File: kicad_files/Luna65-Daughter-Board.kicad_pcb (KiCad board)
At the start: 2 copper layers, 25.1 x 25.1 mm, 29 parts, among them J1 TYPE-C-31-M12_13, J2 Molex Power, J3 JSTPH, J4 Conn_01x03, U1 MCP73831, U2 USBLC6-2SC6, U3 AP2112

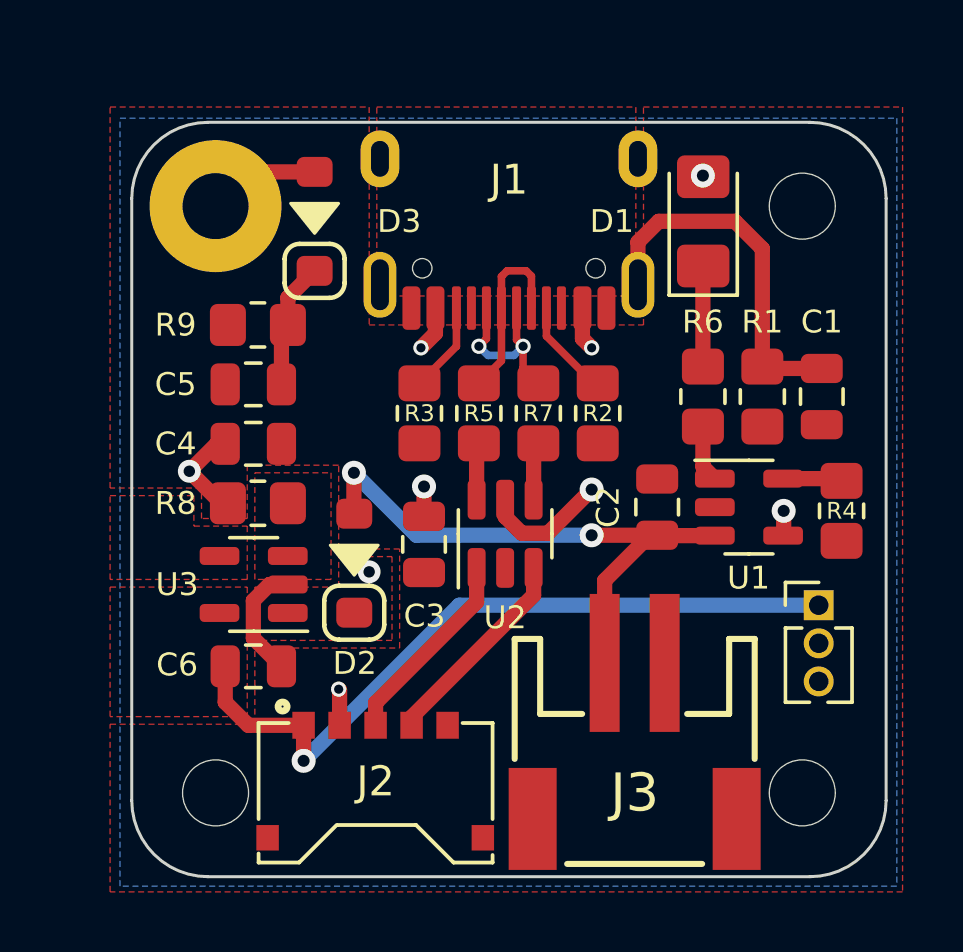
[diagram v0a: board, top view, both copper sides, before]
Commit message: DB Rev B
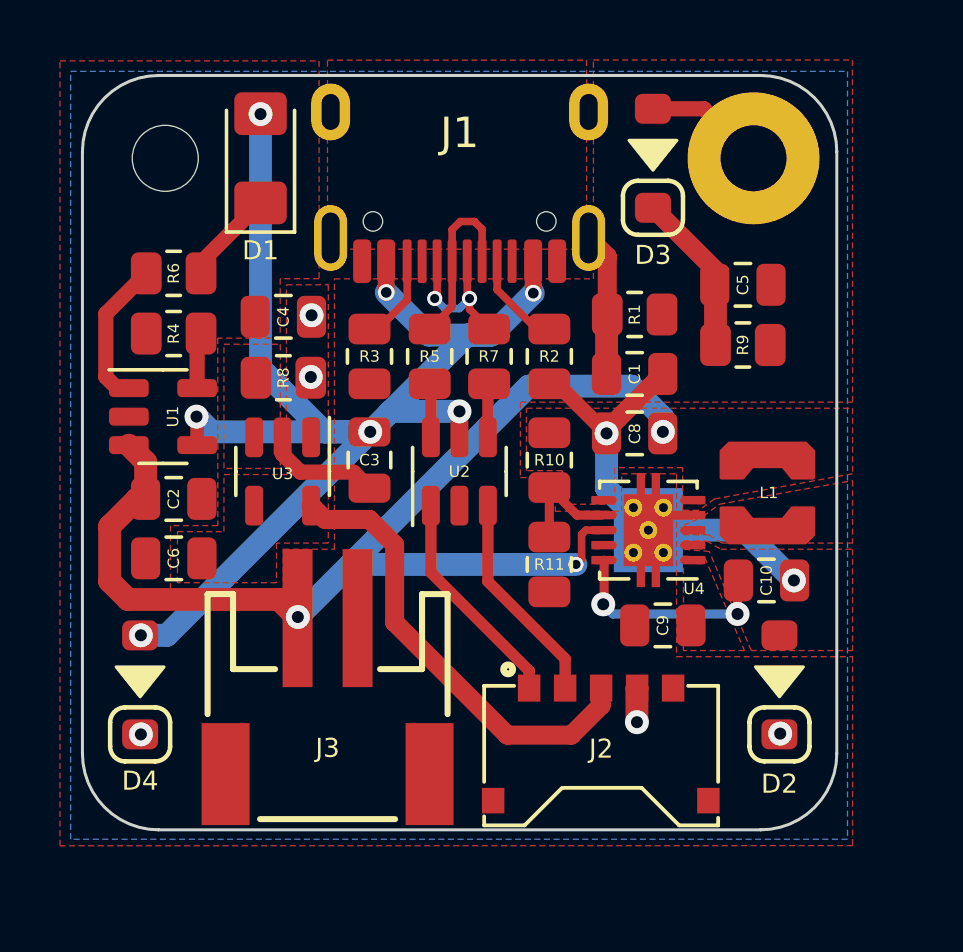
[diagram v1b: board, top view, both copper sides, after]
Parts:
- removed H2, H3: MountingHole, MountingHole:MountingHole_2.2mm_M2
- removed J4: Conn_01x03, Connector_PinHeader_1.27mm:PinHeader_1x03_P1.27mm_Vertical
- added C10: 22uF, acheron_Components:C_0805_2012Metric, F.Cu at (83.5, 37.6)
- added C8: 10uF, acheron_Components:C_0805_2012Metric, F.Cu at (79.1, 32.7)
- added C9: 1uF, acheron_Components:C_0805_2012Metric, F.Cu at (80.0, 39.1)
- added D4: MBR120, acheron_Components:D_SOD-123, F.Cu at (62.6, 41.1)
- added L1: LPS3015-222ML, Luna65:LPS3015, F.Cu at (83.6, 34.7)
- added R10: 3.6M, Resistor_SMD:R_0805_2012Metric, F.Cu at (76.3, 33.6)
- added R11: 261K, Resistor_SMD:R_0805_2012Metric, F.Cu at (76.3, 37.1)
- added U4: TPS61202DRC, Package_SON:Texas_S-PVSON-N10_ThermalVias, F.Cu at (79.6, 36.0)
- R1, R2, R3, R4, R5, R6, R7, R8, R9: footprint Resistor_SMD:R_0805_2012Metric_Pad1.20x1.40mm_HandSolder -> Resistor_SMD:R_0805_2012Metric
- moved R4 23.0 mm to (63.7, 29.4), turned to 180 degrees
- moved H1 21.3 mm to (63.4, 23.6)
- moved U1 19.8 mm to (63.4, 32.2)
- moved R6 18.1 mm to (63.7, 27.4), turned to 0 degrees
- moved H4 18.0 mm to (83.1, 23.6)
- moved C5 16.7 mm to (82.7, 27.8), turned to 0 degrees
- moved R9 16.2 mm to (82.7, 29.8), turned to 180 degrees
- moved C2 16.1 mm to (63.7, 34.9), turned to 180 degrees
- moved D1 14.9 mm to (66.6, 23.6)
- moved D2 14.7 mm to (83.9, 41.1)
- moved D3 11.5 mm to (79.7, 23.6)
- moved J3 10.3 mm to (68.9, 42.6)
- moved J2 7.62 mm to (78.0, 43.1)
- moved C1 6.28 mm to (79.1, 30.8), turned to 180 degrees
- moved R1 5.06 mm to (79.1, 28.8), turned to 0 degrees
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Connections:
- C3 pad 2: VBUS -> VUSB
- C4 pad 1: VBUS -> 5V
- D1 pad 2: VBUS -> VUSB
- D2 pad 1: VBUS -> 5V
- D2 pad 2: VBAT -> Net-(C10-Pad1)
- J1 pad A4: VBUS -> VUSB
- J1 pad B4: VBUS -> VUSB
- J2 pad 1: 3.3V -> D-
- J2 pad 2: VBUS -> D+
- J2 pad 3: D- -> 3.3V
- J2 pad 4: D+ -> 5V
- R8 pad 1: VBUS -> 5V
- U1 pad 4: VBUS -> VUSB
- U2 pad 5: VBUS -> VUSB
- U3 pad 1: VBUS -> 5V
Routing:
- net VUSB: track 0.00 -> 47.2 mm, vias 0 -> 7
- net VBAT: track 19.3 -> 37.6 mm, vias 2 -> 3
- net GND: track 3.95 -> 20.3 mm, vias 0 -> 2
- net VBUS: track 13.6 -> 0.00 mm, vias 9 -> 0
- net 3.3V: track 24.6 -> 15.3 mm, vias 1 -> 0
- net /SHIELD: track 12.2 -> 4.77 mm
- net Net-(C10-Pad1): track 0.00 -> 7.22 mm, vias 0 -> 2
- net Net-(R10-Pad2): track 0.00 -> 3.79 mm
- net Net-(R6-Pad1): track 1.90 -> 4.93 mm
- net Net-(C5-Pad1): track 4.24 -> 5.40 mm
- net 5V: track 0.00 -> 1.14 mm, vias 0 -> 5
- net D-: track 6.64 -> 7.44 mm
- net DBus+: track 5.91 -> 5.29 mm
- added copper zone on B.Cu, net 5V
- added copper zone on F.Cu, net 5V
- added copper zone on F.Cu, net Net-(C10-Pad1)
- added copper zone on F.Cu, net Net-(C9-Pad1)
- added copper zone on F.Cu, net Net-(L1-Pad2)
- added copper zone on F.Cu, net VBAT
- removed copper zone on B.Cu, net VBUS
- removed copper zone on F.Cu, net VBUS
- removed copper zone on F.Cu, net unconnected-(U3-Pad4)

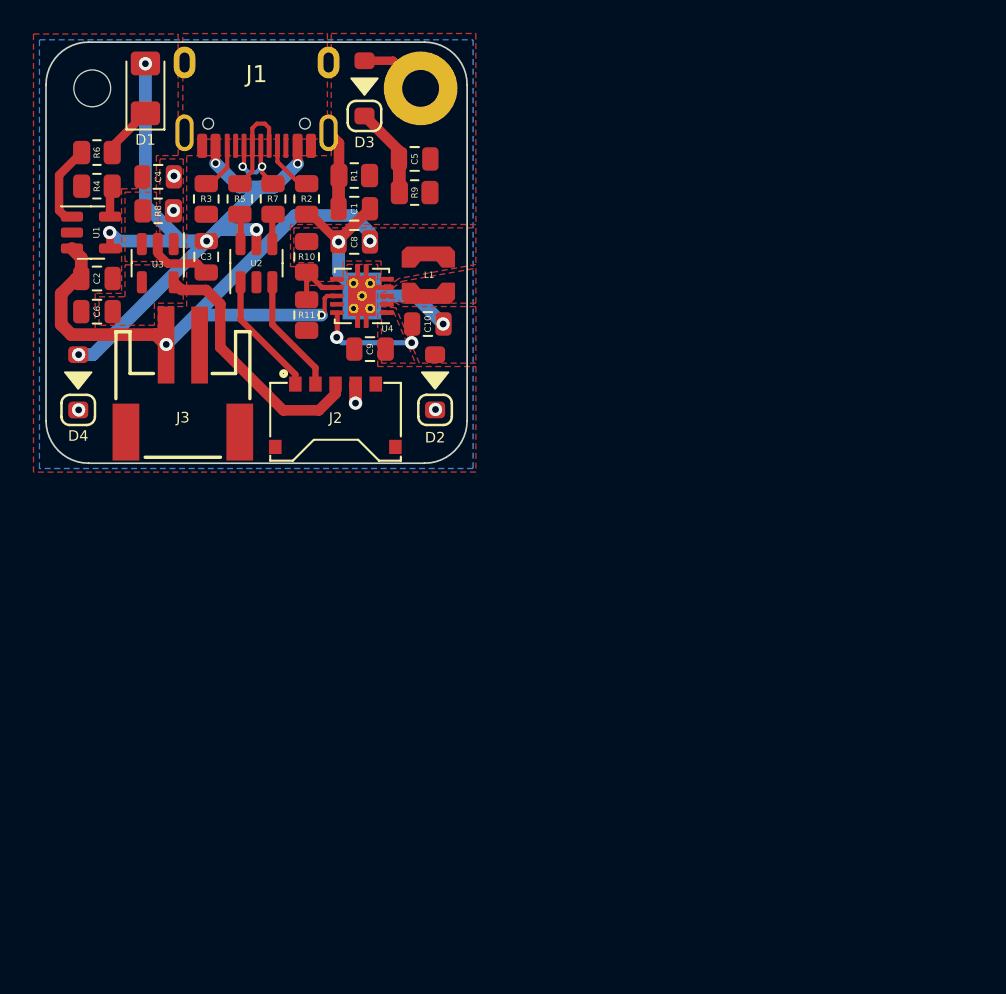
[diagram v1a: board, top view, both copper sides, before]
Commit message: DB Rev C
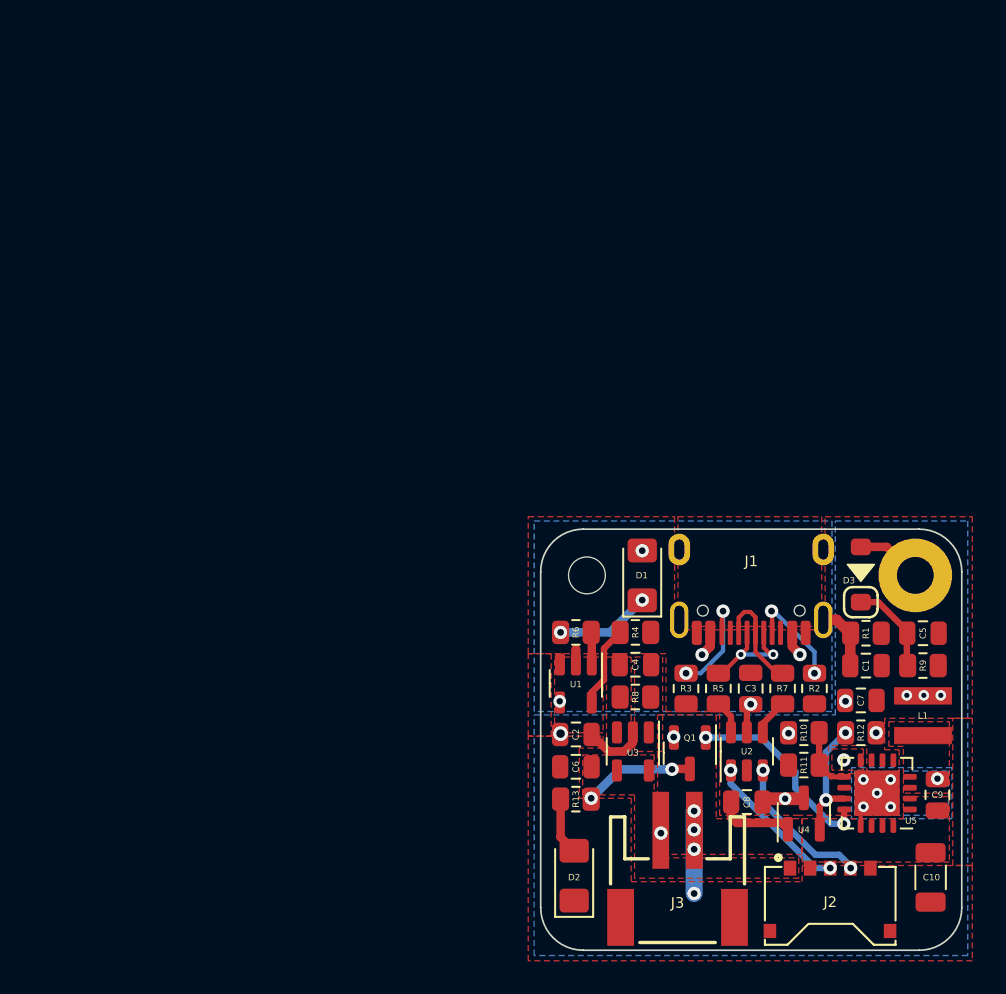
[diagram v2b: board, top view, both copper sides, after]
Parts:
- removed the C9 at (80.0, 39.1)
- removed D4: MBR120, acheron_Components:D_SOD-123
- removed H4: MountingHole, MountingHole:MountingHole_2.2mm_M2_Pad
- added C10: 220uF, Capacitor_SMD:C_1206_3216Metric, F.Cu at (113.5, 70.7)
- added C7: 0.1uF, acheron_Components:C_0805_2012Metric, F.Cu at (109.3, 60.1)
- added H2: MountingHole, MountingHole:MountingHole_2.2mm_M2_Pad, F.Cu at (112.6, 52.7)
- added Q1: MMUN2133LT1G, Package_TO_SOT_SMD:SOT-23, F.Cu at (99.1, 63.3)
- added R12: 100K, Resistor_SMD:R_0805_2012Metric, F.Cu at (109.3, 62.1)
- added R13: 1K, Resistor_SMD:R_0805_2012Metric, F.Cu at (92.3, 66.0)
- added U5: TPS61032RSAR, Package_DFN_QFN:Texas_S-PVQFN-N16_EP2.7x2.7mm, F.Cu at (110.3, 65.7)
- C9: renamed from C10; value 22uF -> 2.2uF
- D2: value MBR120 -> Red; footprint acheron_Components:D_SOD-123 -> LED_SMD:LED_1206_3216Metric_Pad1.42x1.75mm_HandSolder
- J1: value TYPE-C-31-M12_13 -> TYPE-C-31-M12
- L1: value LPS3015-222ML -> 6.8uH XAL4030; footprint Luna65:LPS3015 -> Luna65:XAL4030
- R10: value 3.6M -> 2.34M
- R11: value 261K -> 390K
- R4: value 10K -> 1K
- U4: value TPS61202DRC -> APX803L; footprint Package_SON:Texas_S-PVSON-N10_ThermalVias -> Package_TO_SOT_SMD:SOT-23
- moved R7 42.2 mm to (104.7, 59.4)
- moved R2 42.1 mm to (106.6, 59.4)
- moved R4 41.8 mm to (95.9, 56.1), turned to 0 degrees
- moved D1 41.5 mm to (96.3, 52.7)
- moved C5 41.5 mm to (113.1, 56.1)
- moved C3 41.5 mm to (102.8, 59.4), turned to -90 degrees
- moved D3 41.5 mm to (109.3, 52.6)
- moved R9 41.5 mm to (113.1, 58.0)
- moved H1 41.5 mm to (93.0, 52.7)
- moved J1 41.5 mm to (102.8, 56.8)
- moved C9 41.4 mm to (113.9, 65.8), turned to 90 degrees
- moved J3 41.4 mm to (98.4, 71.6)
- moved J2 41.3 mm to (107.5, 72.0)
- moved U2 41.3 mm to (102.5, 63.2)
- moved R10 41.1 mm to (105.9, 62.1), turned to 0 degrees
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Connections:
- C9 pad 1: Net-(C10-Pad1) -> 5V
- D2 pad 1: 5V -> GND
- D2 pad 2: Net-(C10-Pad1) -> Net-(D2-Pad2)
- J2 pad 1: D- -> 3.3V
- J2 pad 2: D+ -> 5V
- J2 pad 3: 3.3V -> D-
- J2 pad 4: 5V -> D+
- J3 pad NC1: (no net) -> GND
- J3 pad NC2: (no net) -> GND
- U4 pad 1: Net-(C9-Pad1) -> GND
- U4 pad 2: Net-(C10-Pad1) -> /EN
- U4 pad 3: Net-(L1-Pad2) -> VBAT
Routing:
- net VUSB: track 47.2 -> 4.45 mm, vias 7 -> 5
- net VBAT: track 37.6 -> 2.50 mm, vias 3 -> 11
- net 3.3V: track 15.3 -> 0.00 mm
- net /LBO: track 0.00 -> 11.8 mm, vias 0 -> 2
- net /EN: track 0.00 -> 7.52 mm, vias 0 -> 2
- net Net-(C10-Pad1): track 7.22 -> 0.00 mm, vias 2 -> 0
- net Net-(Q1-Pad3): track 0.00 -> 6.62 mm, vias 0 -> 2
- net GND: track 20.3 -> 15.1 mm, vias 2 -> 10
- net Net-(D2-Pad2): track 0.00 -> 3.52 mm
- net Net-(J1-PadB5): track 2.95 -> 6.46 mm, vias 0 -> 2
- net Net-(R6-Pad1): track 4.93 -> 1.82 mm
- net Net-(R4-Pad1): track 1.87 -> 4.84 mm
- net Net-(J1-PadA5): track 3.23 -> 6.16 mm, vias 0 -> 2
- net Net-(D1-Pad1): track 3.17 -> 5.68 mm, vias 0 -> 2
- net D+: track 7.15 -> 8.84 mm, vias 0 -> 2
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- added copper zone on B.Cu, net GND
- added copper zone on B.Cu, net VBAT
- added copper zone on B.Cu, net VUSB
- removed copper zone on B.Cu, net 5V
- removed copper zone on F.Cu, net Net-(C10-Pad1)
- removed copper zone on F.Cu, net Net-(C9-Pad1)
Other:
- rule pad_to_mask_clearance: 0 -> 0.0508
